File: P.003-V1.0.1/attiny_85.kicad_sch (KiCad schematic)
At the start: 3 parts, among them SW2 SW_Push, SW3 SW_Push, U1 ATtiny85-20P

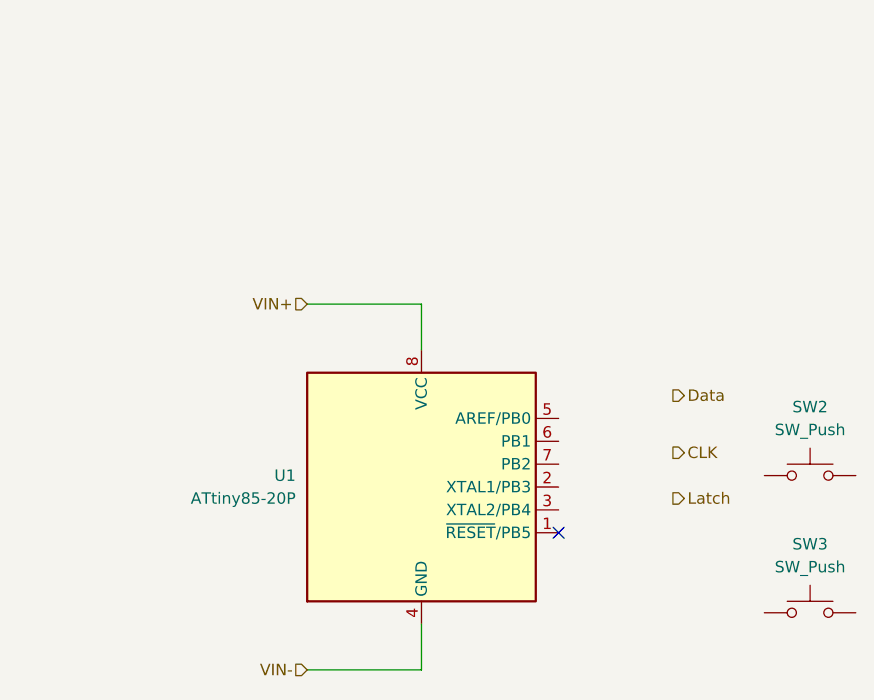
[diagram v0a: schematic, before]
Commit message: Schematic wired
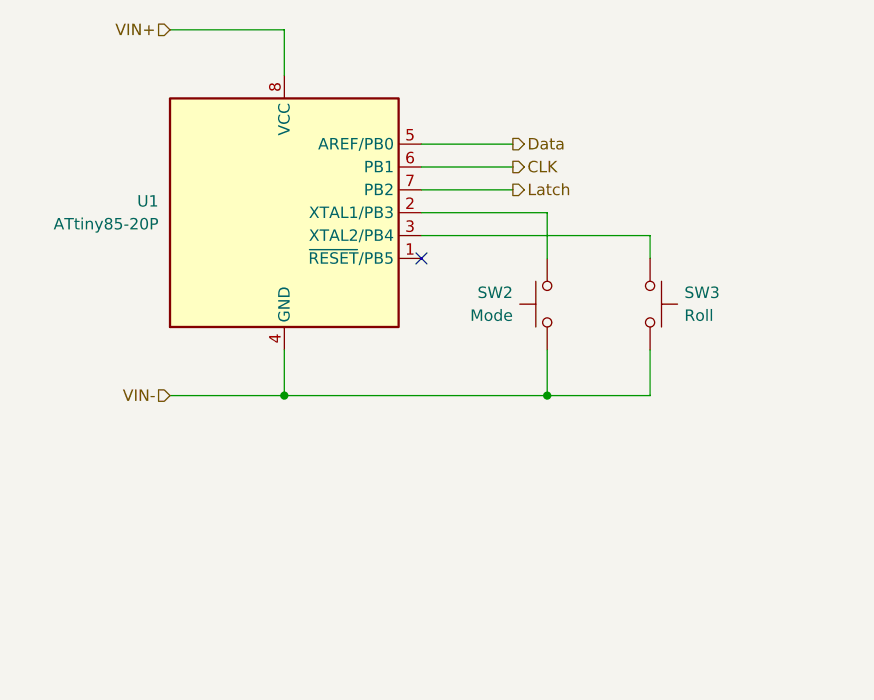
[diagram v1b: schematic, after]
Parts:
- SW2: value SW_Push -> Mode
- SW3: value SW_Push -> Roll
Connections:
- net CLK: now also U1.6 (PB1)
- net Data: now also U1.5 (AREF/PB0)
- net Latch: now also U1.7 (PB2)
- net VIN-: now also SW2.2, SW3.2
- net at SW2.1: now also U1.2 (XTAL1/PB3)
- net at SW3.1: now also U1.3 (XTAL2/PB4)
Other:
- company: (none) -> GSAS - Labs
- title: (none) -> Attiny 85
- moved on the sheet: SW2, SW3, U1
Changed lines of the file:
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@@
 	(generator_version "10.0")
 	(paper "A4")
+	(title_block
+		(title "Attiny 85")
+		(date "2026-08-23")
+		(rev "01")
+		(company "GSAS - Labs")
+	)
+	(junction
+		(at 166.37 116.84)
+		(diameter 0)
+		(color 0 0 0 0)
+	)
+	(junction
+		(at 137.16 116.84)
+		(diameter 0)
+		(color 0 0 0 0)
+	)
 	(no_connect
-		(at 167.64 132.08)
-	)
-	(wire
-		(pts
-			(xy 152.4 147.32) (xy 152.4 142.24)
-		)
-		(stroke
-			(width 0)
-			(type default)
-		)
-	)
-	(wire
-		(pts
-			(xy 139.7 106.68) (xy 152.4 106.68)
-		)
-		(stroke
-			(width 0)
-			(type default)
-		)
-	)
-	(wire
-		(pts
-			(xy 139.7 147.32) (xy 152.4 147.32)
-		)
-		(stroke
-			(width 0)
-			(type default)
-		)
-	)
-	(wire
-		(pts
-			(xy 152.4 106.68) (xy 152.4 111.76)
+		(at 152.4 101.6)
+	)
+	(wire
+		(pts
+			(xy 137.16 111.76) (xy 137.16 116.84)
+		)
+		(stroke
+			(width 0)
+			(type default)
+		)
+	)
+	(wire
+		(pts
+			(xy 152.4 88.9) (xy 162.56 88.9)
+		)
+		(stroke
+			(width 0)
+			(type default)
+		)
+	)
+	(wire
+		(pts
+			(xy 137.16 76.2) (xy 137.16 81.28)
+		)
+		(stroke
+			(width 0)
+			(type default)
+		)
+	)
+	(wire
+		(pts
+			(xy 177.8 99.06) (xy 152.4 99.06)
+		)
+		(stroke
+			(width 0)
+			(type default)
+		)
+	)
+	(wire
+		(pts
+			(xy 137.16 116.84) (xy 166.37 116.84)
+		)
+		(stroke
+			(width 0)
+			(type default)
+		)
+	)
+	(wire
+		(pts
+			(xy 177.8 116.84) (xy 166.37 116.84)
+		)
+		(stroke
+			(width 0)
+			(type default)
+		)
+	)
+	(wire
+		(pts
+			(xy 152.4 93.98) (xy 162.56 93.98)
+		)
+		(stroke
+			(width 0)
+			(type default)
+		)
+	)
+	(wire
+		(pts
+			(xy 166.37 101.6) (xy 166.37 96.52)
+		)
+		(stroke
+			(width 0)
+			(type default)
+		)
+	)
+	(wire
+		(pts
+			(xy 166.37 116.84) (xy 166.37 111.76)
+		)
+		(stroke
+			(width 0)
+			(type default)
+		)
+	)
+	(wire
+		(pts
+			(xy 124.46 76.2) (xy 137.16 76.2)
+		)
+		(stroke
+			(width 0)
+			(type default)
+		)
+	)
+	(wire
+		(pts
+			(xy 124.46 116.84) (xy 137.16 116.84)
+		)
+		(stroke
+			(width 0)
+			(type default)
+		)
+	)
+	(wire
+		(pts
+			(xy 177.8 111.76) (xy 177.8 116.84)
+		)
+		(stroke
+			(width 0)
+			(type default)
+		)
+	)
+	(wire
+		(pts
+			(xy 177.8 101.6) (xy 177.8 99.06)
+		)
+		(stroke
+			(width 0)
+			(type default)
+		)
+	)
+	(wire
+		(pts
+			(xy 152.4 91.44) (xy 162.56 91.44)
+		)
+		(stroke
+			(width 0)
+			(type default)
+		)
+	)
+	(wire
+		(pts
+			(xy 166.37 96.52) (xy 152.4 96.52)
 		)
 		(stroke
@@
 	(hierarchical_label "VIN-"
 		(shape input)
-		(at 139.7 147.32 180)
+		(at 124.46 116.84 180)
 		(effects
 			(font
@@
 	(hierarchical_label "CLK"
 		(shape output)
-		(at 180.34 123.19 0)
+		(at 162.56 91.44 0)
 		(effects
 			(font
@@
 	(hierarchical_label "Data"
 		(shape output)
-		(at 180.34 116.84 0)
+		(at 162.56 88.9 0)
 		(effects
 			(font
@@
 	(hierarchical_label "VIN+"
 		(shape input)
-		(at 139.7 106.68 180)
+		(at 124.46 76.2 180)
 		(effects
 			(font
@@
 	(hierarchical_label "Latch"
 		(shape output)
-		(at 180.34 128.27 0)
+		(at 162.56 93.98 0)
 		(effects
 			(font
@@
 	(symbol
 		(lib_id "Switch:SW_Push")
-		(at 195.58 125.73 0)
+		(at 166.37 106.68 90)
+		(mirror x)
 		(unit 1)
 		(body_style 1)
@@
 		(in_pos_files yes)
 		(dnp no)
-		(fields_autoplaced yes)
 		(property "Reference" "SW2"
-			(at 195.58 118.11 0)
-			(show_name no)
-			(do_not_autoplace no)
-			(effects
-				(font
-					(size 1.27 1.27)
-				)
-			)
-		)
-		(property "Value" "SW_Push"
-			(at 195.58 120.65 0)
-			(show_name no)
-			(do_not_autoplace no)
-			(effects
-				(font
-					(size 1.27 1.27)
-				)
+			(at 162.56 105.4099 90)
+			(show_name no)
+			(do_not_autoplace no)
+			(effects
+				(font
+					(size 1.27 1.27)
+				)
+				(justify left)
+			)
+		)
+		(property "Value" "Mode"
+			(at 162.56 107.9499 90)
+			(show_name no)
+			(do_not_autoplace no)
+			(effects
+				(font
+					(size 1.27 1.27)
+				)
+				(justify left)
 			)
 		)
 		(property "Footprint" ""
-			(at 195.58 120.65 0)
+			(at 161.29 106.68 0)
 			(hide yes)
 			(show_name no)
@@
 		)
 		(property "Datasheet" ""
-			(at 195.58 120.65 0)
+			(at 161.29 106.68 0)
 			(hide yes)
 			(show_name no)
@@
 		)
 		(property "Description" "Push button switch, generic, two pins"
-			(at 195.58 125.73 0)
+			(at 166.37 106.68 0)
 			(hide yes)
 			(show_name no)
@@
 	(symbol
 		(lib_id "Switch:SW_Push")
-		(at 195.58 140.97 0)
+		(at 177.8 106.68 270)
 		(unit 1)
 		(body_style 1)
@@
 		(fields_autoplaced yes)
 		(property "Reference" "SW3"
-			(at 195.58 133.35 0)
-			(show_name no)
-			(do_not_autoplace no)
-			(effects
-				(font
-					(size 1.27 1.27)
-				)
-			)
-		)
-		(property "Value" "SW_Push"
-			(at 195.58 135.89 0)
-			(show_name no)
-			(do_not_autoplace no)
-			(effects
-				(font
-					(size 1.27 1.27)
-				)
+			(at 181.61 105.4099 90)
+			(show_name no)
+			(do_not_autoplace no)
+			(effects
+				(font
+					(size 1.27 1.27)
+				)
+				(justify left)
+			)
+		)
+		(property "Value" "Roll"
+			(at 181.61 107.9499 90)
+			(show_name no)
+			(do_not_autoplace no)
+			(effects
+				(font
+					(size 1.27 1.27)
+				)
+				(justify left)
 			)
 		)
 		(property "Footprint" ""
-			(at 195.58 135.89 0)
+			(at 182.88 106.68 0)
 			(hide yes)
 			(show_name no)
@@
 		)
 		(property "Datasheet" ""
-			(at 195.58 135.89 0)
+			(at 182.88 106.68 0)
 			(hide yes)
 			(show_name no)
@@
 		)
 		(property "Description" "Push button switch, generic, two pins"
-			(at 195.58 140.97 0)
+			(at 177.8 106.68 0)
 			(hide yes)
 			(show_name no)
@@
 	(symbol
 		(lib_id "MCU_Microchip_ATtiny:ATtiny85-20P")
-		(at 152.4 127 0)
+		(at 137.16 96.52 0)
 		(unit 1)
 		(body_style 1)
@@
 		(fields_autoplaced yes)
 		(property "Reference" "U1"
-			(at 138.43 125.7299 0)
+			(at 123.19 95.2499 0)
 			(show_name no)
 			(do_not_autoplace no)
@@
 		)
 		(property "Value" "ATtiny85-20P"
-			(at 138.43 128.2699 0)
+			(at 123.19 97.7899 0)
 			(show_name no)
 			(do_not_autoplace no)
@@
 		)
 		(property "Footprint" "Package_DIP:DIP-8_W7.62mm"
-			(at 152.4 127 0)
+			(at 137.16 96.52 0)
 			(hide yes)
 			(show_name no)
@@
 		)
 		(property "Datasheet" "http://ww1.microchip.com/downloads/en/DeviceDoc/atmel-2586-avr-8-bit-microcontroller-attiny25-attiny45-attiny85_datasheet.pdf"
-			(at 152.4 127 0)
+			(at 137.16 96.52 0)
 			(hide yes)
 			(show_name no)
@@
 		)
 		(property "Description" "20MHz, 8kB Flash, 512B SRAM, 512B EEPROM, debugWIRE, DIP-8"
-			(at 152.4 127 0)
-			(hide yes)
-			(show_name no)
+			(at 137.16 96.52 0)
+			(hide yes)
+			(show_name no)

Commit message: add footprint
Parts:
- SW2, SW3: footprint (none) -> Button_Switch_THT:SW_PUSH-12mm
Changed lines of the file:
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@@
 			)
 		)
-		(property "Footprint" ""
+		(property "Footprint" "Button_Switch_THT:SW_PUSH-12mm"
 			(at 161.29 106.68 0)
 			(hide yes)
@@
 			)
 		)
-		(property "Footprint" ""
+		(property "Footprint" "Button_Switch_THT:SW_PUSH-12mm"
 			(at 182.88 106.68 0)
 			(hide yes)
